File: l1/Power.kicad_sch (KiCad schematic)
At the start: 20 parts, among them IC1 LM2587S-ADJ

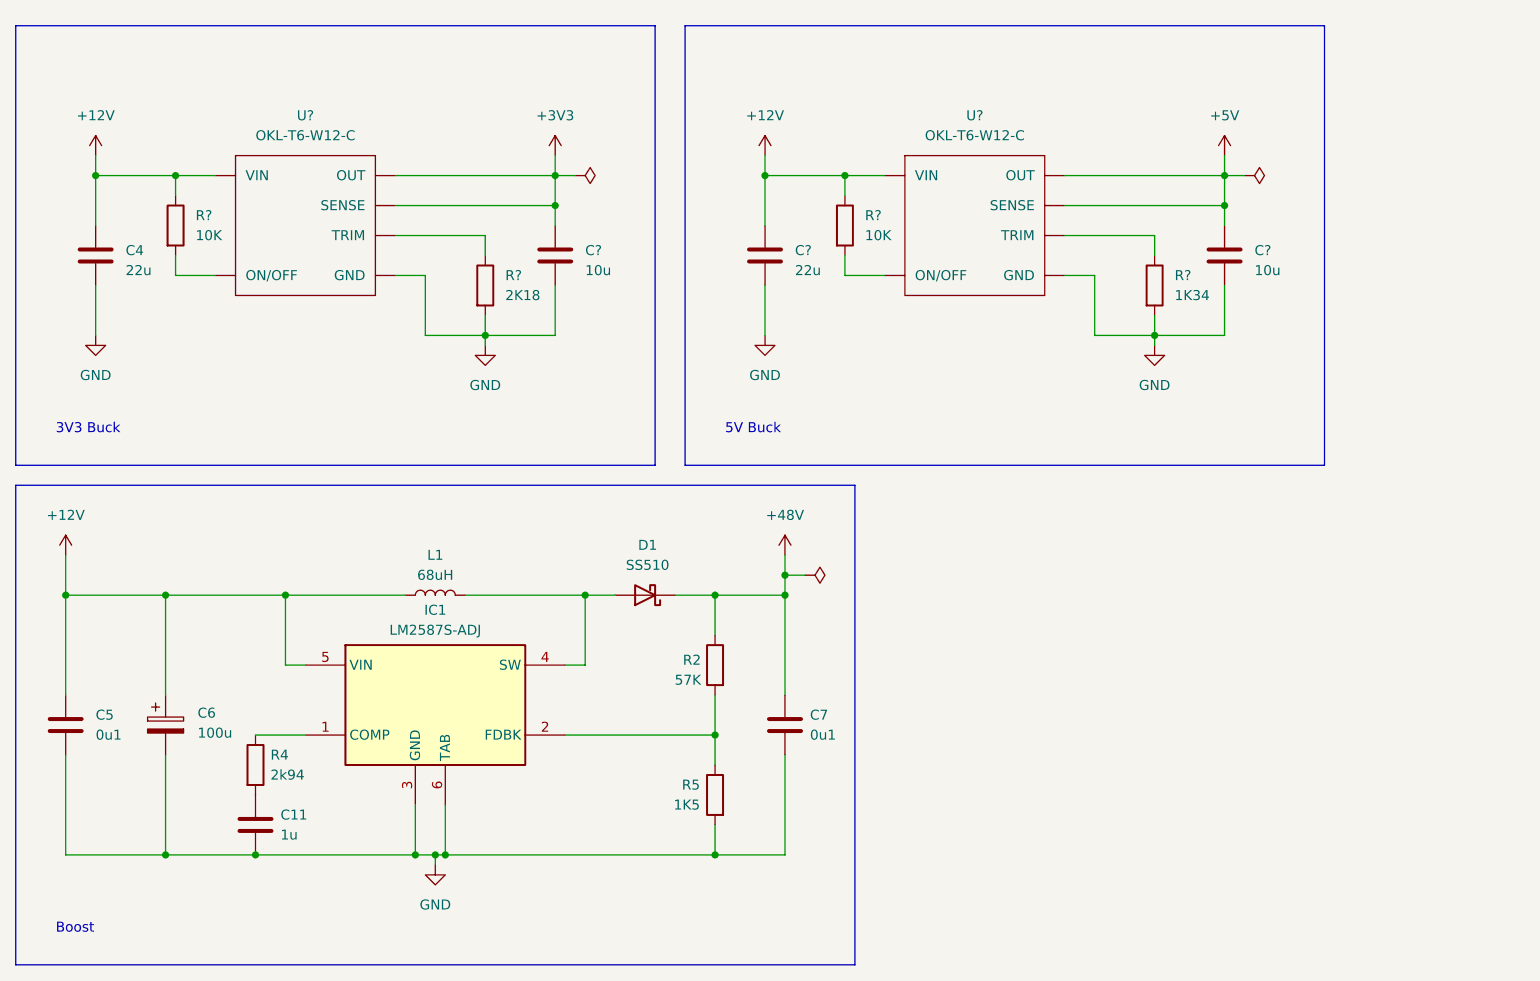
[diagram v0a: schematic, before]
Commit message: Changed To OKL
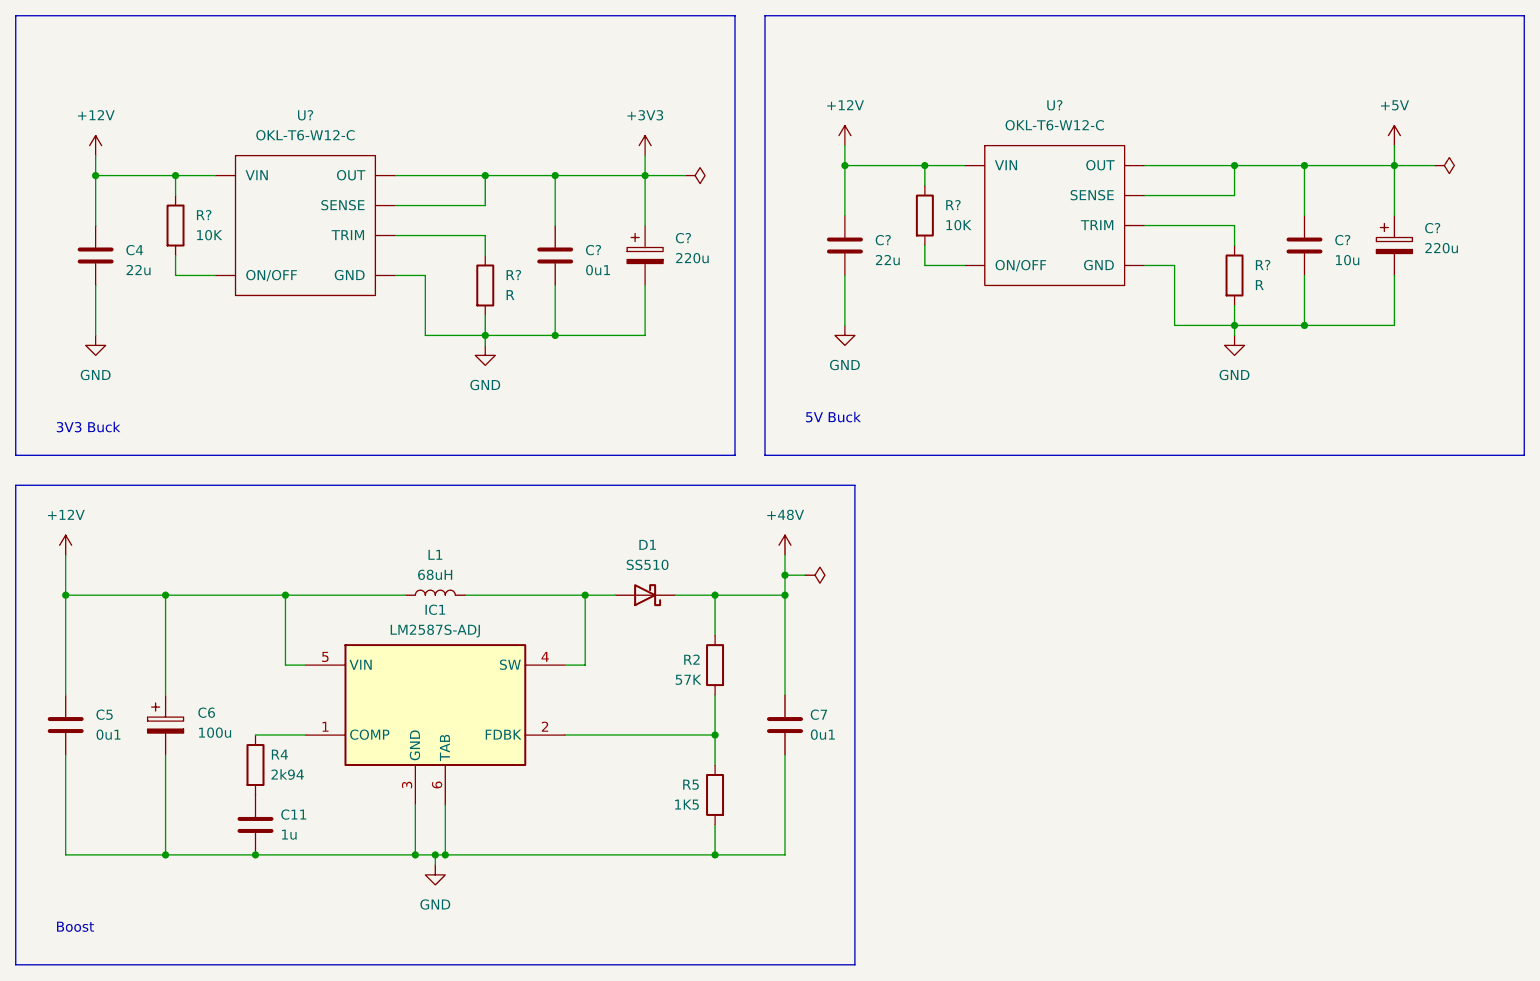
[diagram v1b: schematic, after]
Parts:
- added C? (x2): 220u, symbol Device:C_Polarized
- C?: value 10u -> 0u1
- R?: value 2K18 -> R
- R?: value 1K34 -> R
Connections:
- net +3V3: now also C?.1
- net +5V: now also C?.1
- net GND: now also C?.2, C?.2
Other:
- moved on the sheet: C?, R?, U?
